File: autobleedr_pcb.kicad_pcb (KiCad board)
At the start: 2 copper layers, 91 x 78.5 mm, 13 parts, among them J1 Barrel_Jack, J2 Conn_01x13_Pin, J3 Conn_01x14_Pin, J5 Conn_01x05_Pin, J6 Conn_01x05_Pin, J7 Screw_Terminal_01x02, J8 Conn_01x02_Pin, J9 Conn_01x02_Pin, U1 ESP32, U2 TMC2209, U3 Buck Converter, U4 DRV8874

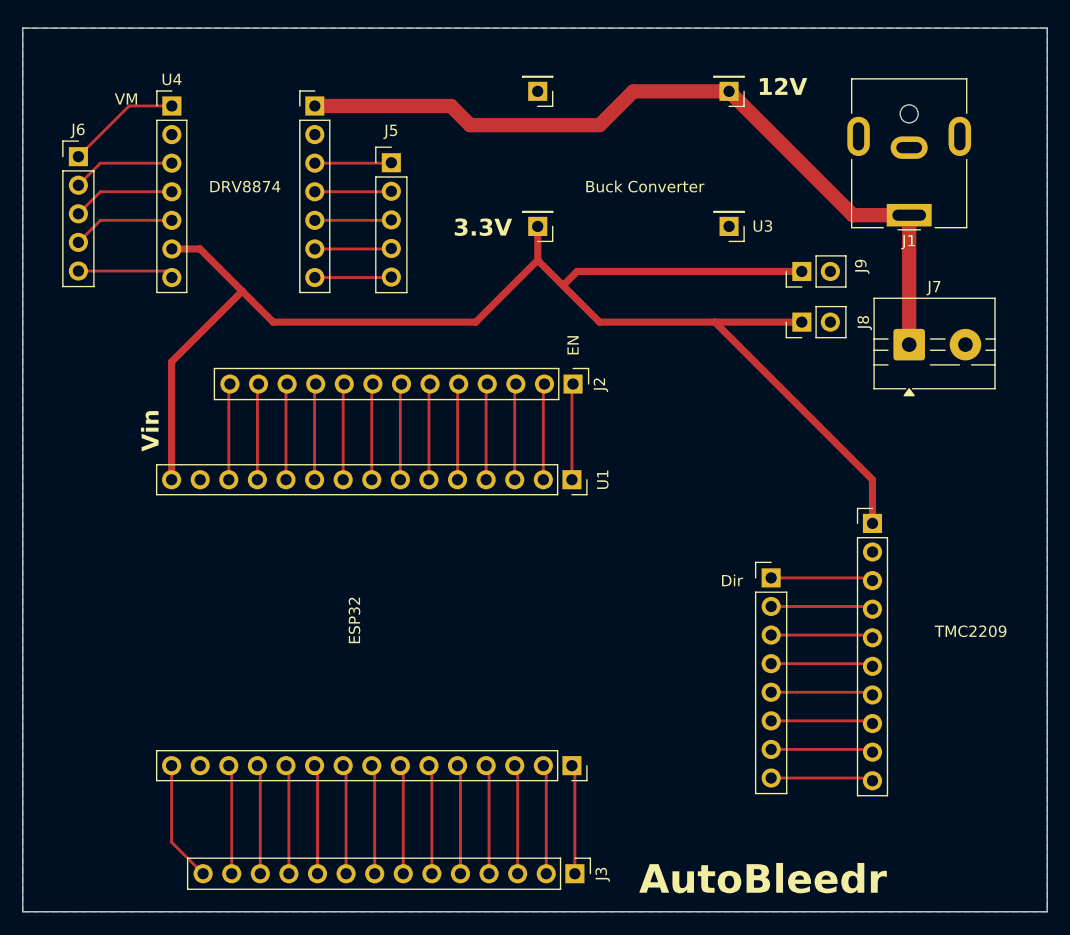
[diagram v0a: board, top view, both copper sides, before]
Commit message: resubmit update 1
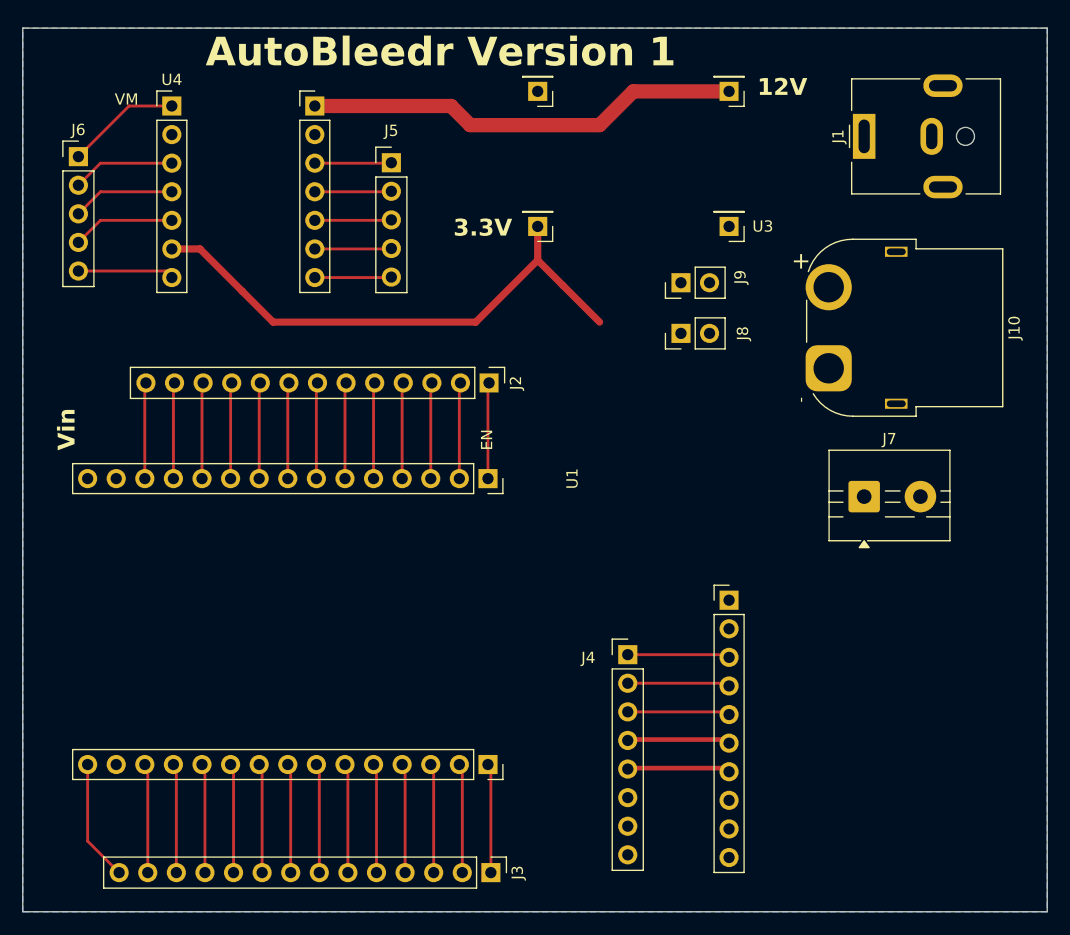
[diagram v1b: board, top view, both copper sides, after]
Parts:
- added J10: XT60 Connector, Connector_AMASS:AMASS_XT60PW-F_1x02_P7.20mm_Horizontal, F.Cu at (141.8, 93.1)
- U1: value ESP32 -> ~
- U2: value TMC2209 -> ~
- U3: value Buck Converter -> ~
- U4: value DRV8874 -> ~
- moved J4 14.5 mm to (124.0, 118.5)
- moved U2 14.5 mm to (133.0, 123.9)
- moved J7 14.1 mm to (145.0, 104.5)
- moved J8 10.8 mm to (128.7, 90.0)
- moved J9 10.8 mm to (128.7, 85.5)
- moved J1 8.06 mm to (145.0, 72.5), turned to 90 degrees
- moved U1 7.46 mm to (111.6, 102.9)
- moved J2 7.46 mm to (111.7, 94.4)
- moved J3 7.46 mm to (111.8, 137.9)
- renumbered Dir to J4
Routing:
- net +3.3V: track 131.3 -> 48.6 mm
- net +12V: track 70.8 -> 38.7 mm
- net Net-(J4-Pin_4): track 9.10 -> 18.2 mm
- net Net-(J4-Pin_8): track 9.10 -> 0.00 mm
- net Net-(J4-Pin_7): track 9.10 -> 0.00 mm
- net Net-(J4-Pin_5): track 9.10 -> 18.2 mm
- net Net-(J4-Pin_6): track 9.10 -> 0.00 mm
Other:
- board text added: "AutoBleedr Version 1"
- board text removed: "AutoBleedr"
